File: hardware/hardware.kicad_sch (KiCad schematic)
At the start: 0 parts

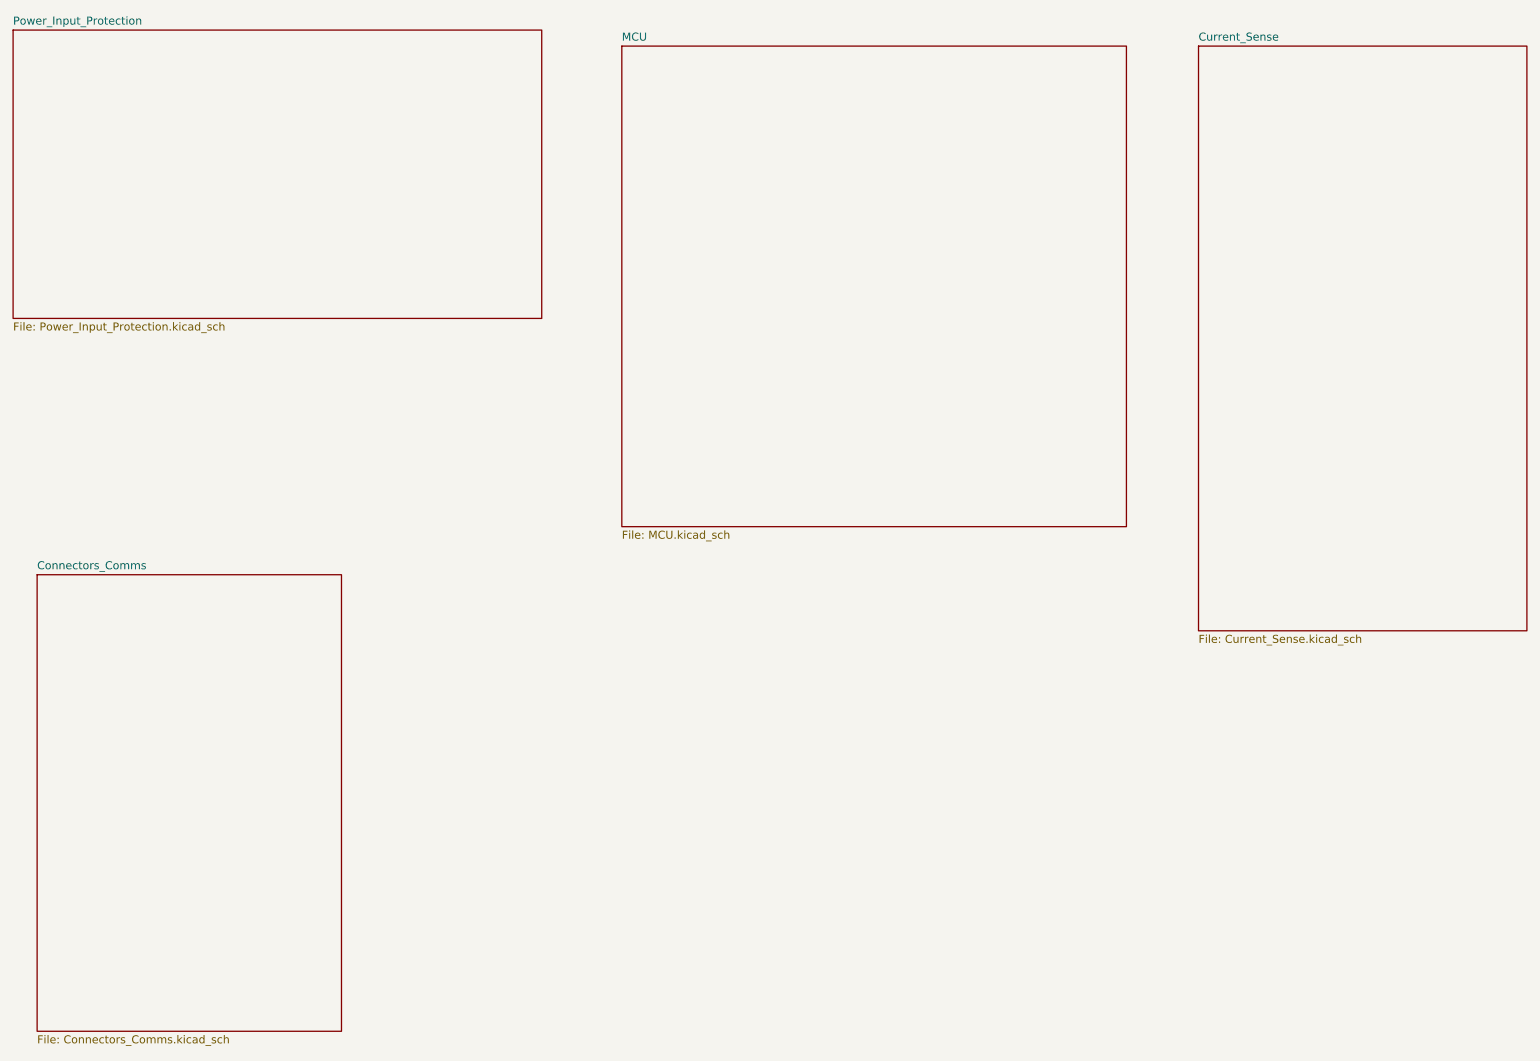
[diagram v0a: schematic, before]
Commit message: Schematics Completed
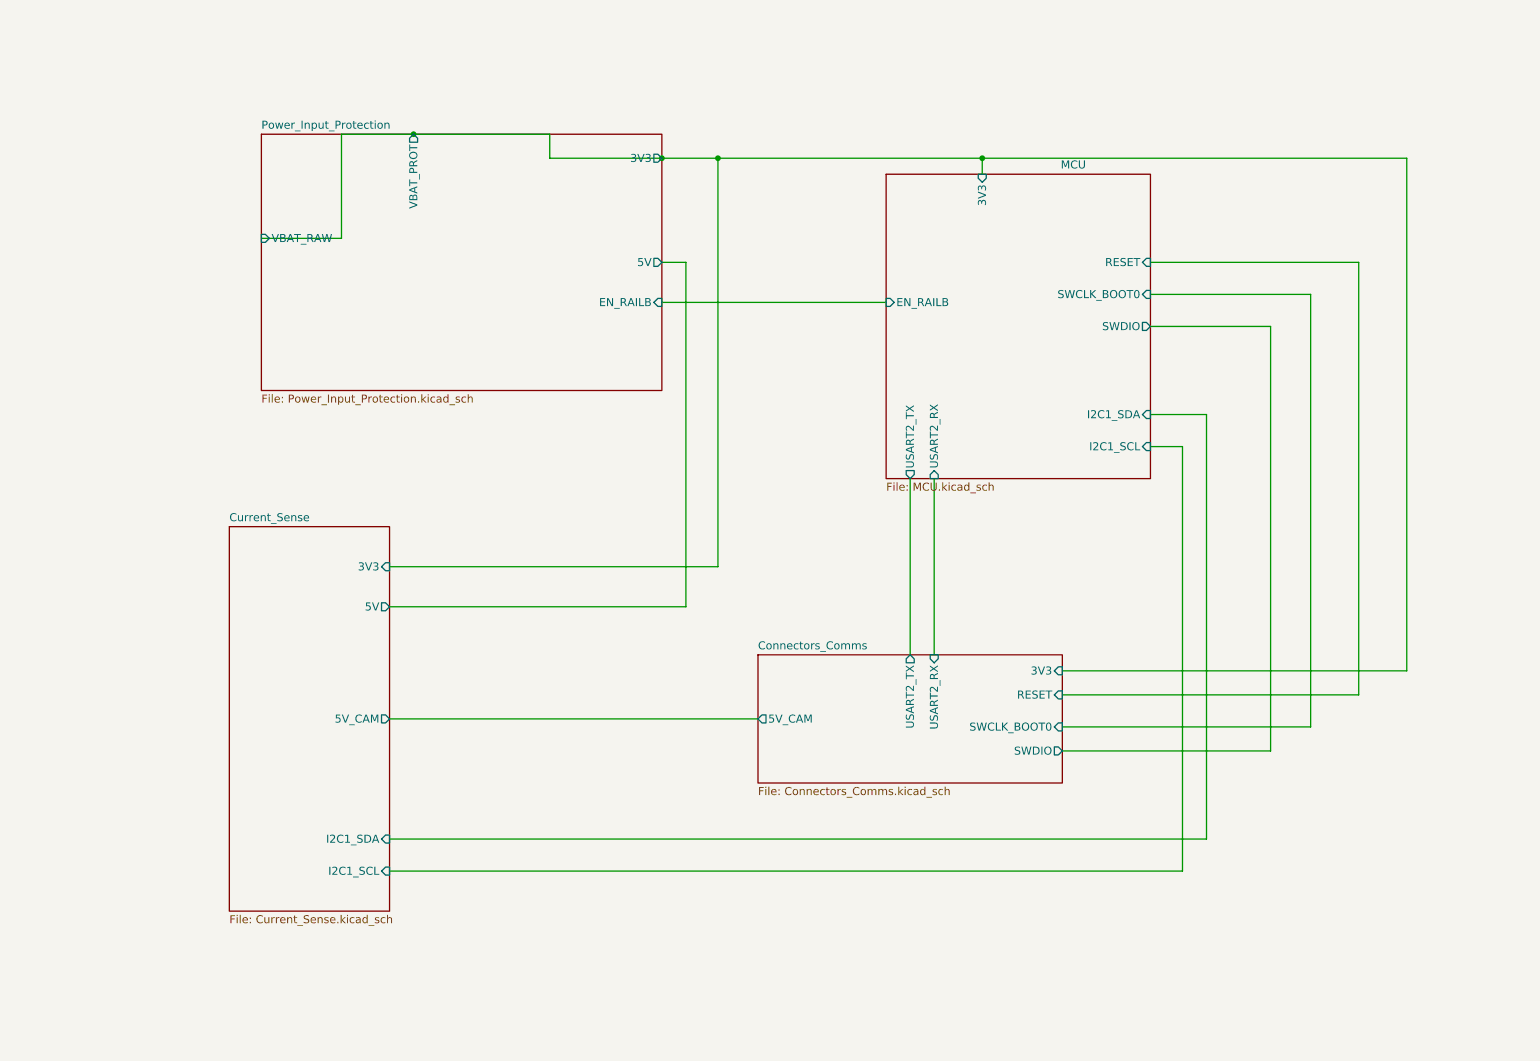
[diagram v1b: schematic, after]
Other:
- sheet Connectors_Comms ports: added 3V3, 5V_CAM, RESET, SWCLK_BOOT0, SWDIO, USART2_RX, USART2_TX; removed none
- sheet Current_Sense ports: added 3V3, 5V, 5V_CAM, I2C1_SCL, I2C1_SDA; removed none
- sheet MCU ports: added 3V3, EN_RAILB, I2C1_SCL, I2C1_SDA, RESET, SWCLK_BOOT0, SWDIO, USART2_RX, USART2_TX; removed none
- sheet Power_Input_Protection ports: added 3V3, 5V, EN_RAILB, VBAT_PROT, VBAT_RAW; removed none
